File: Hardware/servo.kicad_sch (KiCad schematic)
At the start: 3 parts, among them J3 ServoConnector1

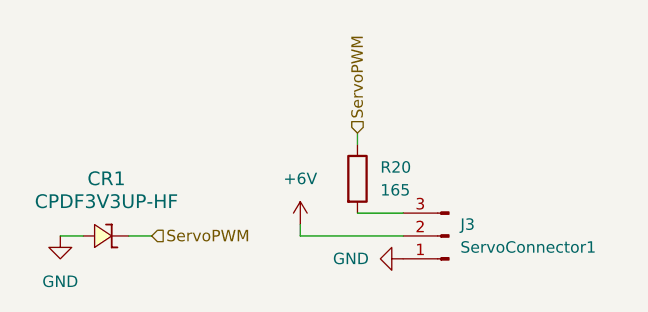
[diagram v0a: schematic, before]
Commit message: tiny tweaks and ready to order
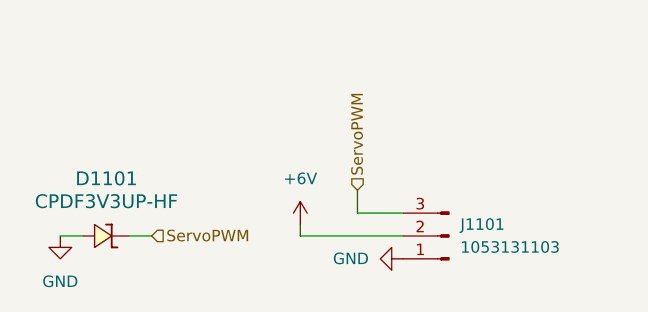
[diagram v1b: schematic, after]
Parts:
- removed R20: 165, Resistor_SMD:R_0402_1005Metric, symbol Device:R
- J1101: renamed from J3; value ServoConnector1 -> 1053131103
- renumbered CR1 to D1101
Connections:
- net ServoPWM: now also J1101.3 (Pin_3)
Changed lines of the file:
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@@
 	(wire
 		(pts
-			(xy 191.77 62.23) (xy 191.77 63.5)
+			(xy 191.77 68.58) (xy 191.77 71.12)
 		)
 		(stroke
@@
 	(hierarchical_label "ServoPWM"
 		(shape input)
-		(at 191.77 62.23 90)
+		(at 191.77 68.58 90)
 		(effects
 			(font
@@
 		(dnp no)
 		(fields_autoplaced yes)
-		(property "Reference" "J3"
+		(property "Reference" "J1101"
 			(at 203.2 72.3899 0)
 			(effects
@@
 			)
 		)
-		(property "Value" "ServoConnector1"
+		(property "Value" "1053131103"
 			(at 203.2 74.9299 0)
 			(effects
@@
 		)
 		(instances
-			(project ""
-				(path "/7db990e4-92e1-4f99-b4d2-435bbec1ba83/55ab0687-c91f-4545-a2ea-e93947dc2af8"
-					(reference "J3")
-					(unit 1)
-				)
-			)
-		)
-	)
-	(symbol
-		(lib_id "Device:R")
-		(at 191.77 67.31 0)
-		(unit 1)
-		(exclude_from_sim no)
-		(in_bom yes)
-		(on_board yes)
-		(dnp no)
-		(fields_autoplaced yes)
-		(property "Reference" "R20"
-			(at 194.31 66.0399 0)
-			(effects
-				(font
-					(size 1.27 1.27)
-				)
-				(justify left)
-			)
-		)
-		(property "Value" "165"
-			(at 194.31 68.5799 0)
-			(effects
-				(font
-					(size 1.27 1.27)
-				)
-				(justify left)
-			)
-		)
-		(property "Footprint" "Resistor_SMD:R_0402_1005Metric"
-			(at 189.992 67.31 90)
-			(effects
-				(font
-					(size 1.27 1.27)
-				)
-				(hide yes)
-			)
-		)
-		(property "Datasheet" "~"
-			(at 191.77 67.31 0)
-			(effects
-				(font
-					(size 1.27 1.27)
-				)
-				(hide yes)
-			)
-		)
-		(property "Description" "Resistor"
-			(at 191.77 67.31 0)
-			(effects
-				(font
-					(size 1.27 1.27)
-				)
-				(hide yes)
-			)
-		)
-		(pin "1"
-		)
-		(pin "2"
-		)
-		(instances
-			(project ""
-				(path "/7db990e4-92e1-4f99-b4d2-435bbec1ba83/55ab0687-c91f-4545-a2ea-e93947dc2af8"
-					(reference "R20")
+			(project "Heimdall"
+				(path "/7db990e4-92e1-4f99-b4d2-435bbec1ba83/55ab0687-c91f-4545-a2ea-e93947dc2af8"
+					(reference "J1101")
 					(unit 1)
 				)
@@
 		(dnp no)
 		(fields_autoplaced yes)
-		(property "Reference" "#PWR051"
+		(property "Reference" "#PWR01103"
 			(at 190.5 76.2 0)
 			(effects
@@
 		)
 		(instances
-			(project ""
-				(path "/7db990e4-92e1-4f99-b4d2-435bbec1ba83/55ab0687-c91f-4545-a2ea-e93947dc2af8"
-					(reference "#PWR051")
+			(project "Heimdall"
+				(path "/7db990e4-92e1-4f99-b4d2-435bbec1ba83/55ab0687-c91f-4545-a2ea-e93947dc2af8"
+					(reference "#PWR01103")
 					(unit 1)
 				)
@@
 		(dnp no)
 		(fields_autoplaced yes)
-		(property "Reference" "#PWR049"
+		(property "Reference" "#PWR01101"
 			(at 158.75 80.01 0)
 			(effects
@@
 		)
 		(instances
-			(project "Reggie"
-				(path "/7db990e4-92e1-4f99-b4d2-435bbec1ba83/55ab0687-c91f-4545-a2ea-e93947dc2af8"
-					(reference "#PWR049")
+			(project "Heimdall"
+				(path "/7db990e4-92e1-4f99-b4d2-435bbec1ba83/55ab0687-c91f-4545-a2ea-e93947dc2af8"
+					(reference "#PWR01101")
 					(unit 1)
 				)
@@
 		(dnp no)
 		(fields_autoplaced yes)
-		(property "Reference" "CR1"
+		(property "Reference" "D1101"
 			(at 163.8808 67.31 0)
 			(effects
@@
 		)
 		(instances
-			(project ""
-				(path "/7db990e4-92e1-4f99-b4d2-435bbec1ba83/55ab0687-c91f-4545-a2ea-e93947dc2af8"
-					(reference "CR1")
+			(project "Heimdall"
+				(path "/7db990e4-92e1-4f99-b4d2-435bbec1ba83/55ab0687-c91f-4545-a2ea-e93947dc2af8"
+					(reference "D1101")
 					(unit 1)
 				)
@@
 		(dnp no)
 		(fields_autoplaced yes)
-		(property "Reference" "#PWR050"
+		(property "Reference" "#PWR01102"
 			(at 185.42 76.2 0)
 			(effects
@@
 		)
 		(instances
-			(project ""
-				(path "/7db990e4-92e1-4f99-b4d2-435bbec1ba83/55ab0687-c91f-4545-a2ea-e93947dc2af8"
-					(reference "#PWR050")
-					(unit 1)
-				)
+			(project "Heimdall"
+				(path "/7db990e4-92e1-4f99-b4d2-435bbec1ba83/55ab0687-c91f-4545-a2ea-e93947dc2af8"
+					(reference "#PWR01102")
+					(unit 1)
+				)
